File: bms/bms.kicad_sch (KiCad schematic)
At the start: 27 parts, among them J10 Conn_02x08_Odd_Even, J11 Conn_02x10_Odd_Even, J13 Conn_02x08_Odd_Even, J14 Conn_02x08_Odd_Even, J2 Conn_01x08_Socket, J22 Conn_02x10_Odd_Even, J3 Conn_01x06_Socket, J5 Conn_01x10_Socket, J6 Conn_01x06_Socket

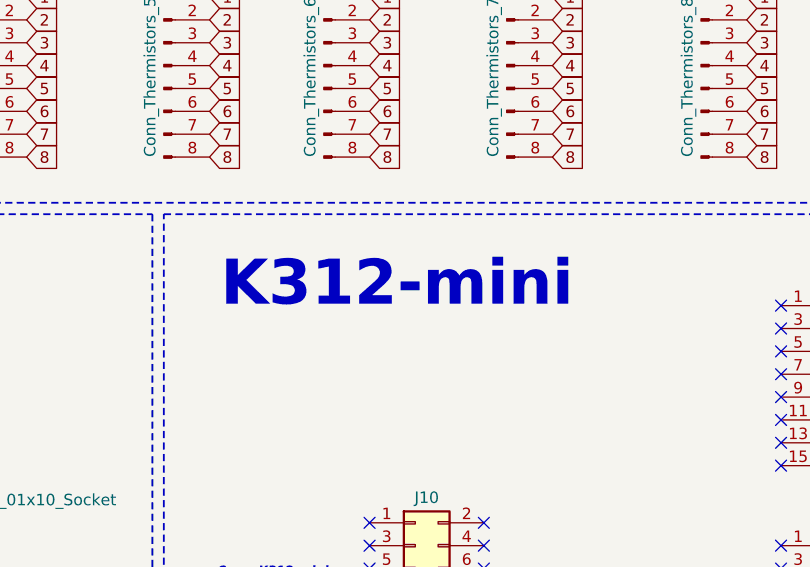
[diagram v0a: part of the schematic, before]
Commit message: fara program deschis
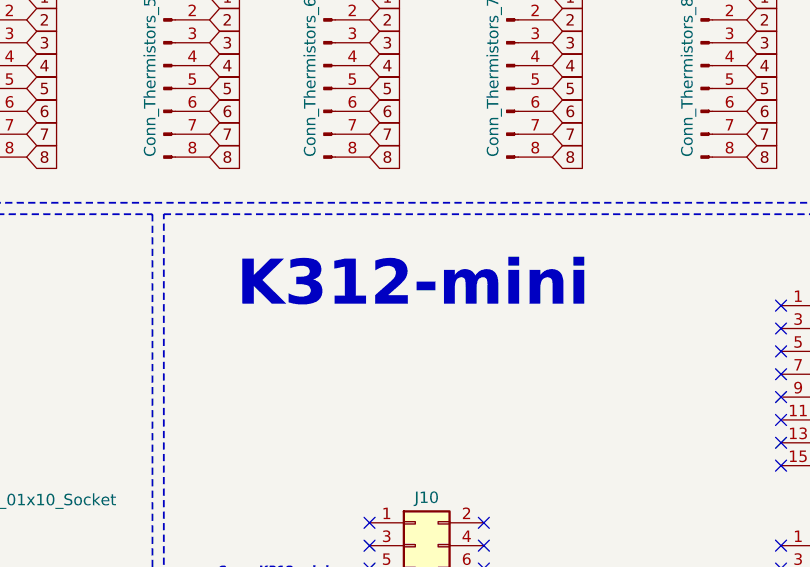
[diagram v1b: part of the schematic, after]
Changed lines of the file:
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@@
 	(text "K312-mini\n"
 		(exclude_from_sim no)
-		(at 124.968 58.674 0)
+		(at 126.746 58.674 0)
 		(effects
 			(font

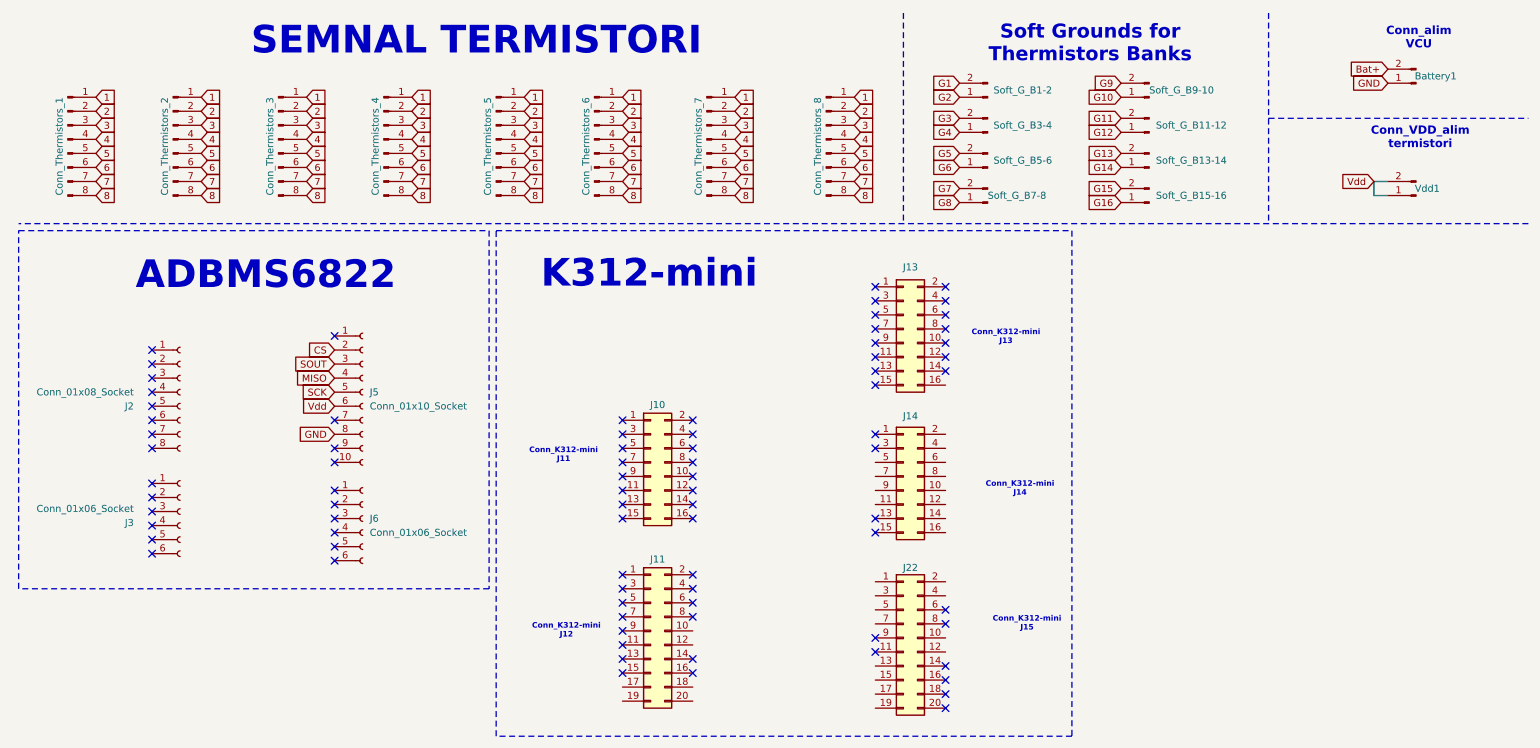
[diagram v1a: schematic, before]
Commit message: v0.99
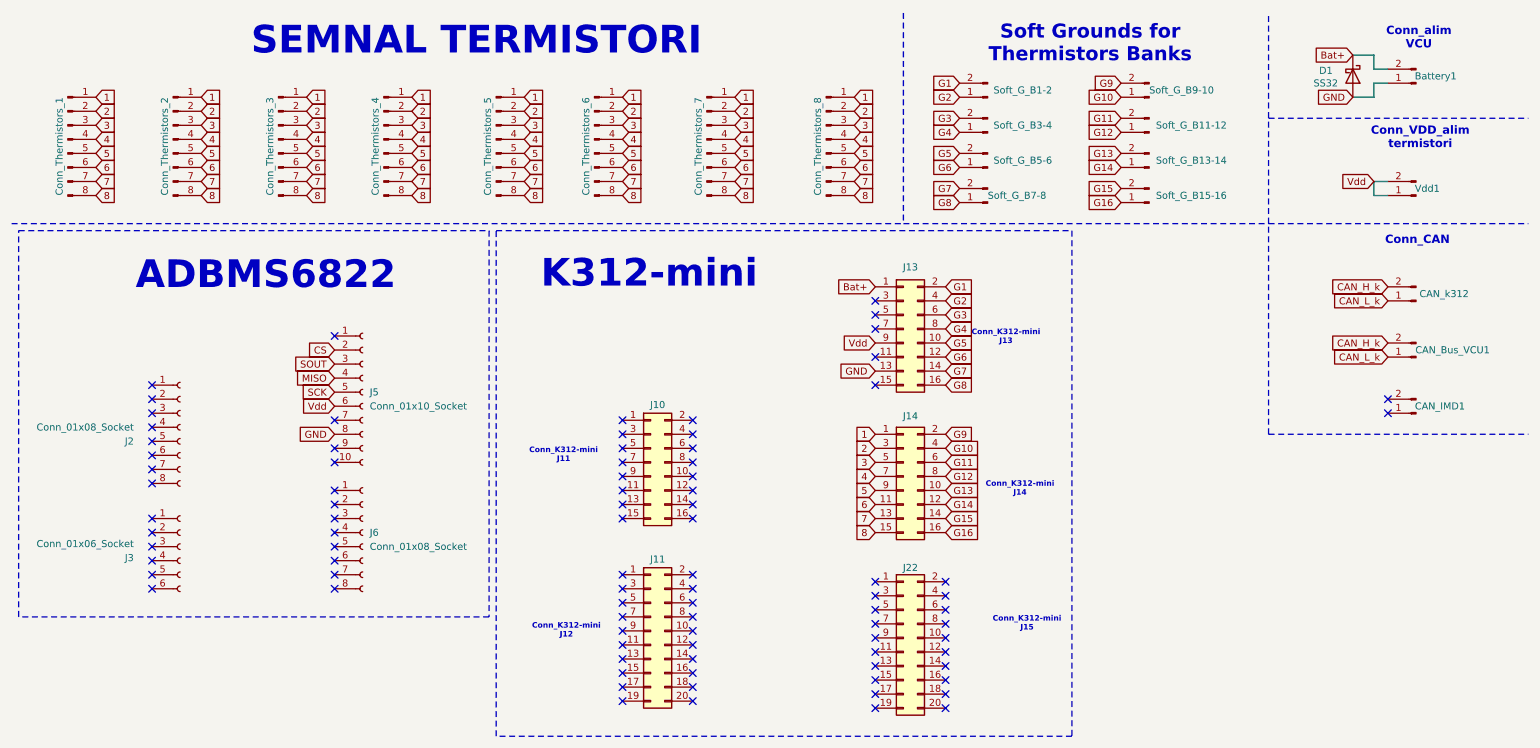
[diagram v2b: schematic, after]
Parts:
- added CAN_Bus_VCU1: Conn_01x02_Pin, Connector_PinHeader_2.00mm:PinHeader_1x02_P2.00mm_Vertical, symbol Connector:Conn_01x02_Pin
- added CAN_IMD1: Conn_01x02_Pin, symbol Connector:Conn_01x02_Pin
- added CAN_k312: Conn_01x02_Pin, Connector_PinHeader_2.54mm:PinHeader_1x02_P2.54mm_Vertical, symbol Connector:Conn_01x02_Pin
- added D1: SS32, Diode_SMD:D_SMB, symbol Diode:SS32
- J6: value Conn_01x06_Socket -> Conn_01x08_Socket; footprint Connector_PinSocket_2.54mm:PinSocket_1x06_P2.54mm_Vertical -> Connector_PinSocket_2.54mm:PinSocket_1x08_P2.54mm_Vertical; symbol Connector:Conn_01x06_Socket -> Connector:Conn_01x08_Socket
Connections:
- net 1: now also J14.1 (Pin_1)
- net 2: now also J14.3 (Pin_3)
- net 3: now also J14.5 (Pin_5)
- net 4: now also J14.7 (Pin_7)
- net 5: now also J14.9 (Pin_9)
- net 6: now also J14.11 (Pin_11)
- net 7: now also J14.13 (Pin_13)
- net 8: now also J14.15 (Pin_15)
- net Bat+: now also J13.1 (Pin_1), D1.1 (K)
- net G1: now also J13.2 (Pin_2)
- net G10: now also J14.4 (Pin_4)
- net G11: now also J14.6 (Pin_6)
- net G12: now also J14.8 (Pin_8)
- net G13: now also J14.10 (Pin_10)
- net G14: now also J14.12 (Pin_12)
- net G15: now also J14.14 (Pin_14)
- net G16: now also J14.16 (Pin_16)
- net G2: now also J13.4 (Pin_4)
- net G3: now also J13.6 (Pin_6)
- net G4: now also J13.8 (Pin_8)
- net G5: now also J13.10 (Pin_10)
- net G6: now also J13.12 (Pin_12)
- net G7: now also J13.14 (Pin_14)
- net G8: now also J13.16 (Pin_16)
- net G9: now also J14.2 (Pin_2)
- net GND: now also J13.13 (Pin_13), D1.2 (A)
- net Vdd: now also J13.9 (Pin_9)
- new net CAN_H_k: CAN_Bus_VCU1.2 (Pin_2), CAN_k312.2 (Pin_2)
- new net CAN_L_k: CAN_Bus_VCU1.1 (Pin_1), CAN_k312.1 (Pin_1)
- no-connect marks 81 -> 89
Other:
- note added: "Conn_CAN"
- moved on the sheet: J2, J3
